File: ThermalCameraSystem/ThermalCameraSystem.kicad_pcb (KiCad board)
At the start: 2 copper layers, 3 parts, among them U1 MLX90621ESF-BAB-000-SP

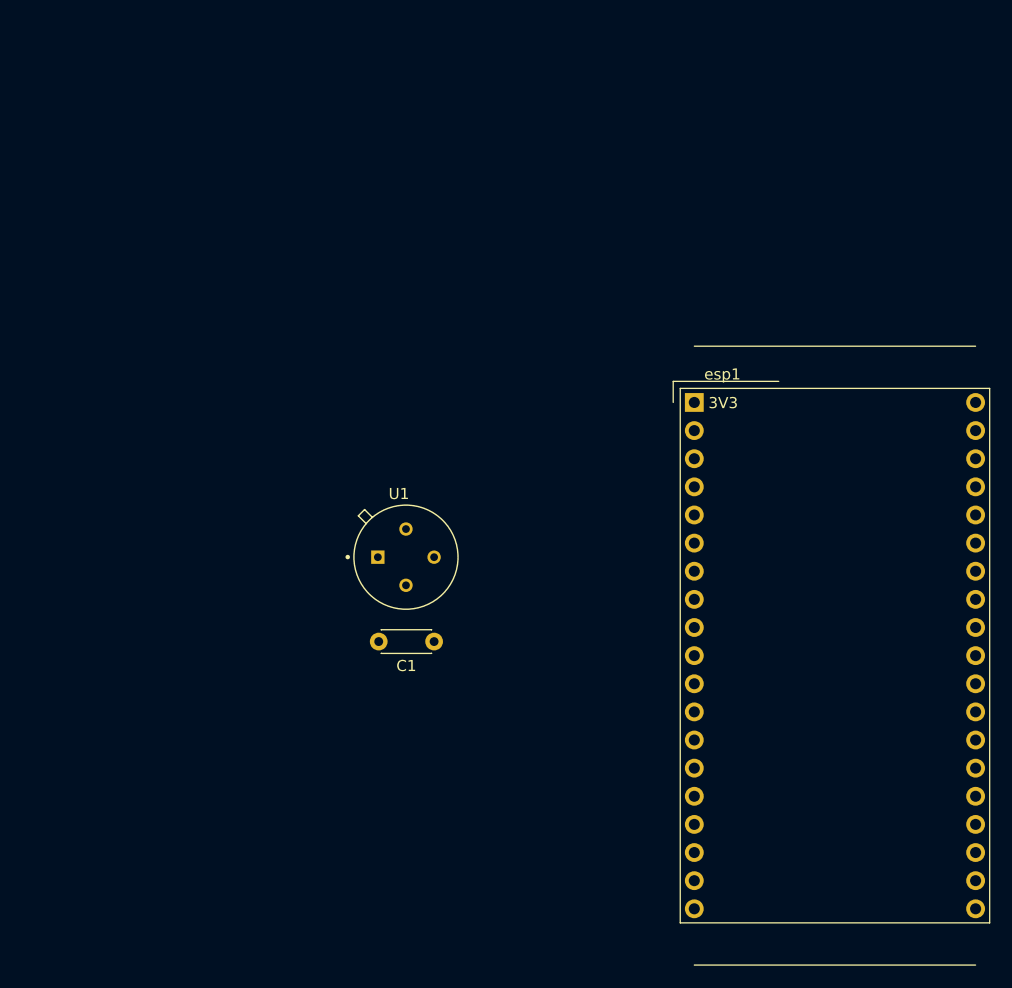
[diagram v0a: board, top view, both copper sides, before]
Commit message: Updated main
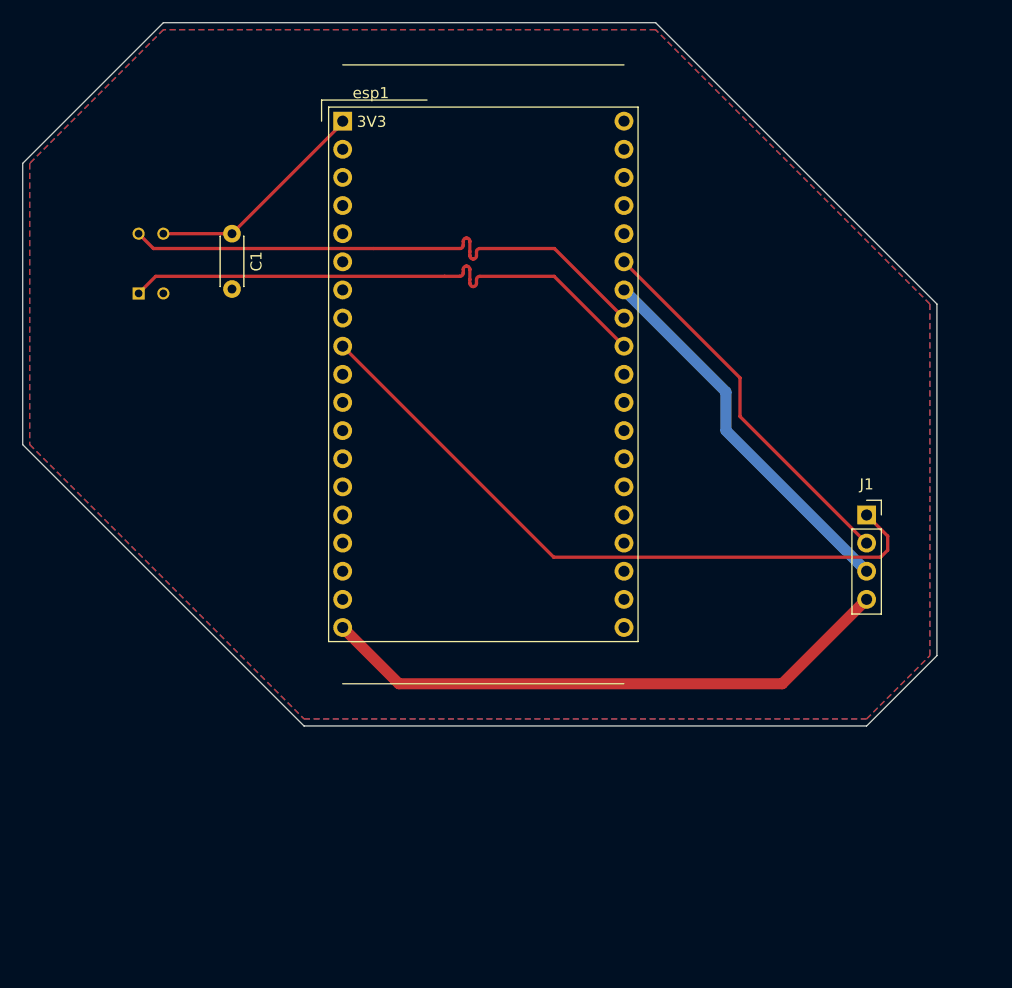
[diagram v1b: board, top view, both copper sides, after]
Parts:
- added J1: Conn_01x04, Connector_PinSocket_2.54mm:PinSocket_1x04_P2.54mm_Vertical, F.Cu at (174.3, 99.1)
- U1: footprint TO254P940H1340-4:TO254P940H1340-4 -> Library:TO292P930H600-4; moved to B.Cu
- moved C1 41.1 mm to (117.0, 73.7), turned to -90 degrees
- moved esp1 40.7 mm to (139.7, 83.8)
- moved U1 35.1 mm to (109.7, 76.4), turned to 180 degrees
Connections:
- esp1 pad 19: unconnected-(esp1-5V-Pad19) -> +5V
- esp1 pad 25: unconnected-(esp1-G21-Pad25) -> BatteryLatch
- esp1 pad 26: GND -> GND1
- esp1 pad 27: unconnected-(esp1-G19-Pad27) -> MLX_SDA
- esp1 pad 28: unconnected-(esp1-G18-Pad28) -> MLX_SCL
- esp1 pad 7: MLX_SCL -> unconnected-(esp1-ADC1_4_G32-Pad7)
- esp1 pad 8: MLX_SDA -> unconnected-(esp1-ADC1_5_G33-Pad8)
- esp1 pad 9: unconnected-(esp1-G25-Pad9) -> BatteryLevel
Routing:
- net BatteryLevel: track 0.00 -> 61.3 mm
- net +5V: track 0.00 -> 52.6 mm
- net MLX_SDA: track 0.00 -> 49.9 mm
- net MLX_SCL: track 0.00 -> 49.9 mm
- net GND1: track 0.00 -> 34.5 mm
- net BatteryLatch: track 0.00 -> 34.5 mm
- net +3.3V: track 0.00 -> 20.5 mm
- added copper zone on B.Cu, net GND
- added copper zone on F.Cu, net GND
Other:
- board outline added: 82.5 x 63.5 mm
